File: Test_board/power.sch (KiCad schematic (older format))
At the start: 22 parts, among them J10 4.19mmBananaJack, J11 4.19mmBananaJack, J12 4.19mmBananaJack, J13 4.19mmBananaJack, J14 USB_OTG, U3 LT3652, U4 LT3652, U5 LTC3113

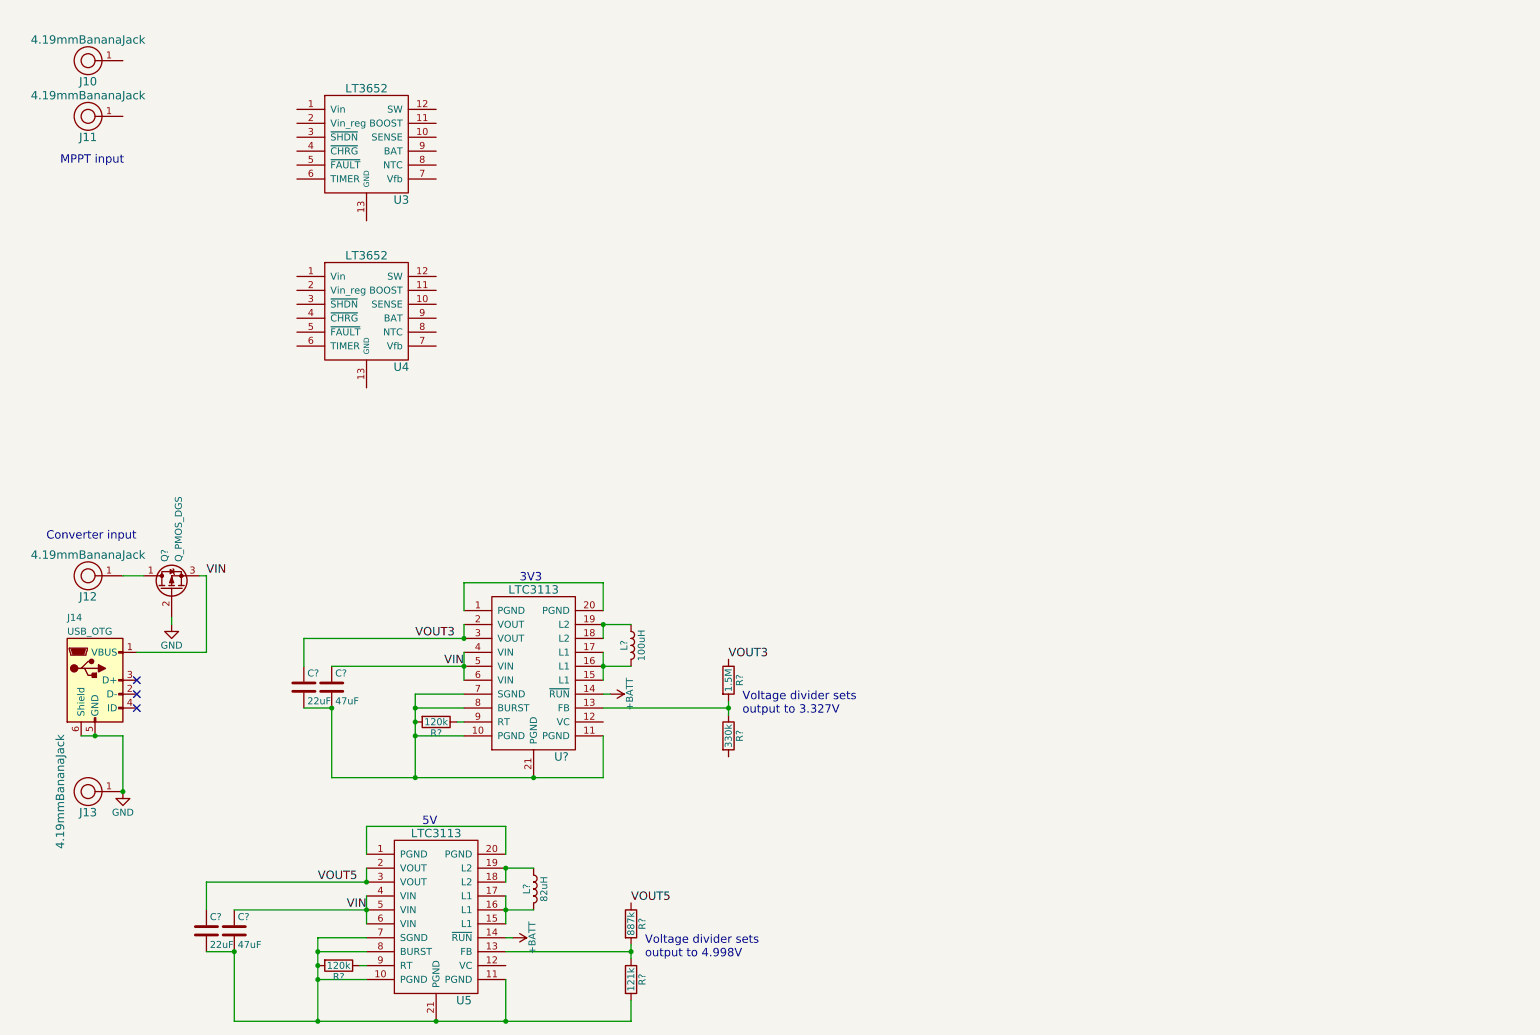
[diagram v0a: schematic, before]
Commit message: Finished schematic
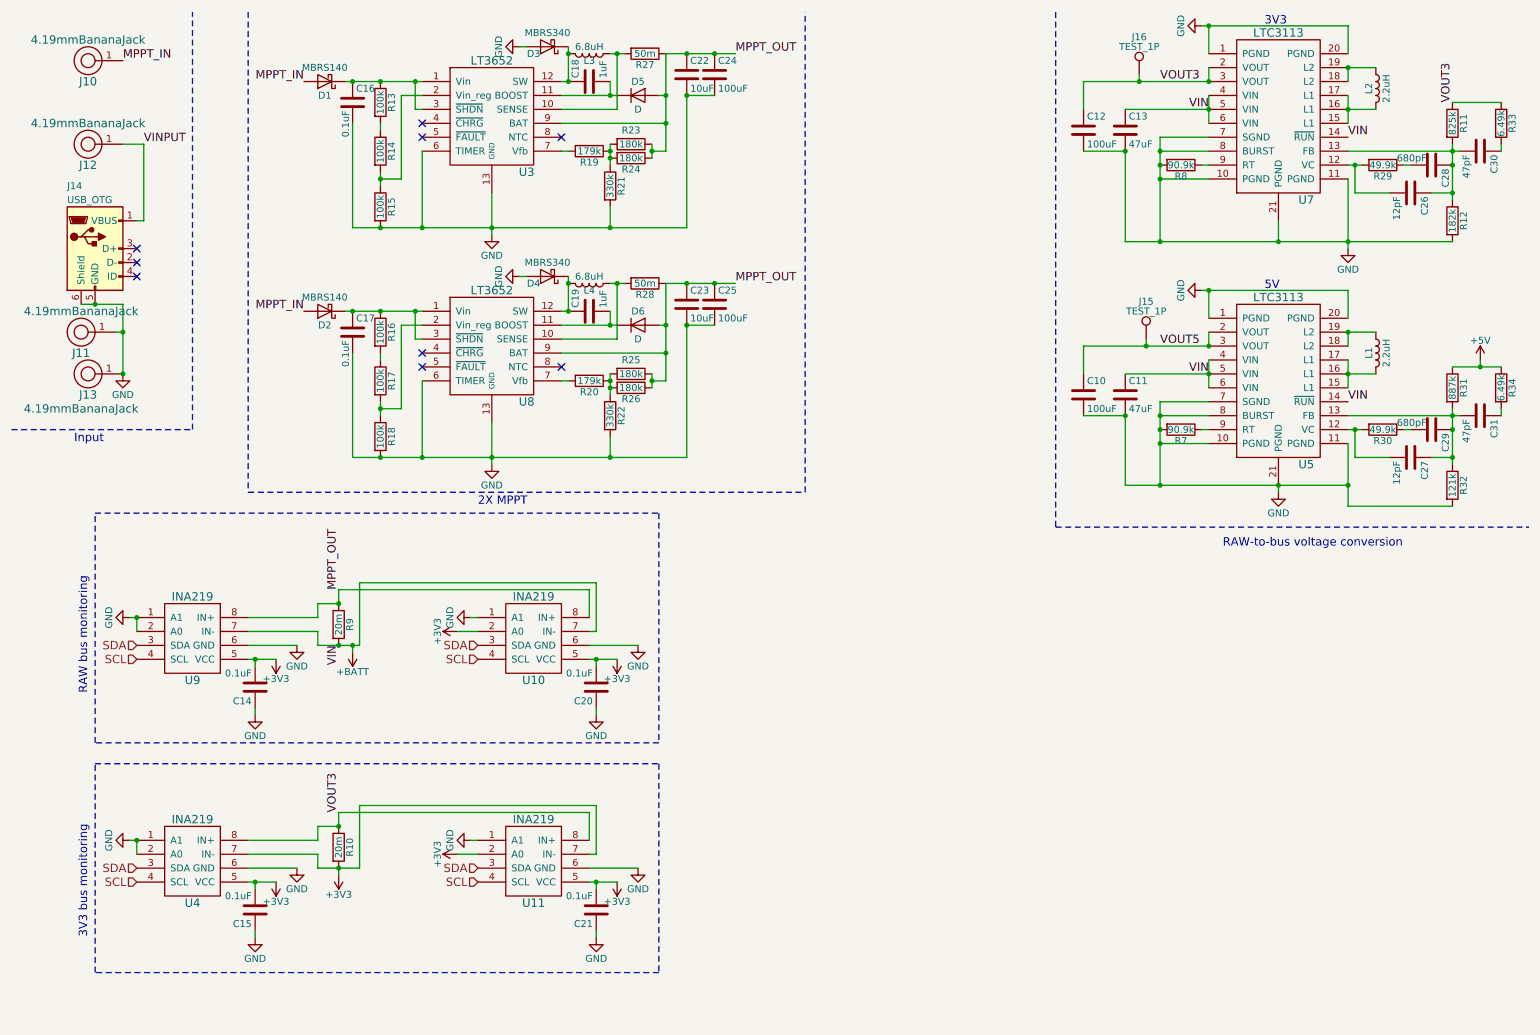
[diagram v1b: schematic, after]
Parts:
- removed Q?: Q_PMOS_DGS, symbol Q_PMOS_DGS
- removed R?: 887k, symbol R
- removed R?: 121k, symbol R
- removed U4: LT3652, symbol LT3652
- added C14, C15, C16, C17, C20, C21: 0.1uF, Capacitors_SMD:C_0805_HandSoldering, symbol C
- added C18, C19: 1uF, symbol C
- added C22, C23: 10uF, symbol C
- added C24, C25: 100uF, symbol C
- added C26, C27: 12pF, symbol C
- added C28, C29: 680pF, symbol C
- added C30, C31: 47pF, symbol C
- added D1, D2: MBRS140, symbol D_Schottky
- added D3, D4: MBRS340, symbol D_Schottky
- added D5, D6: D, symbol D
- added J15, J16: TEST_1P, Measurement_Points:Measurement_Point_Round-SMD-Pad_Big, symbol TEST_1P
- added L3, L4: 6.8uH, symbol L
- added R10, R9: 20m, symbol R
- added R13, R14, R15, R16, R17, R18: 100k, symbol R
- added R19, R20: 179k, symbol R
- added R21, R22: 330k, symbol R
- added R23, R24, R25, R26: 180k, symbol R
- added R27, R28: 50m, symbol R
- added R29, R30: 49.9k, symbol R
- added R31: 887k, symbol R
- added R32: 121k, symbol R
- added R33, R34: 6.49k, symbol R
- added U10, U11, U4, U9: INA219, symbol INA219
- added U8: LT3652, symbol LT3652
- C10, C12: renamed from C?; value 22uF -> 100uF
- L1: renamed from L?; value 82uH -> 2.2uH
- L2: renamed from L?; value 100uH -> 2.2uH
- R11: renamed from R?; value 1.5M -> 825k
- R12: renamed from R?; value 330k -> 182k
- R7, R8: renamed from R?; value 120k -> 90.9k; footprint 0805 -> (none)
- gave numbers to parts that had none: 3
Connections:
- net +BATT: now also C11.1, C13.1, U5.4 (VIN), U5.5 (VIN), U5.6 (VIN), U7.4 (VIN), U7.5 (VIN), U7.6 (VIN), R9.2, U10.7 (IN-), U9.7 (IN-)
- net GND: now also C10.2, C11.2, C12.2, C13.2, J11.1, R12.2, R7.2, R8.2, U3.13 (GND), U3.6 (TIMER), U5.1 (PGND), U5.10 (PGND), U5.11 (PGND), U5.20 (PGND), U5.21 (PGND), U5.7 (SGND), U5.8 (BURST), U7.1 (PGND), U7.10 (PGND), U7.11 (PGND), U7.20 (PGND), U7.21 (PGND), U7.7 (SGND), U7.8 (BURST), C14.1, C15.1, C16.2, C17.2, C20.1, C21.1, C22.2, C23.2, C24.2, C25.2, D3.2 (A), D4.2 (A), R15.2, R18.2, R21.2, R22.2, R32.2, U10.1 (A1), U10.6 (GND), U11.1 (A1), U11.6 (GND), U4.1 (A1), U4.2 (A0), U4.6 (GND), U8.13 (GND), U8.6 (TIMER), U9.1 (A1), U9.2 (A0), U9.6 (GND)
- net VOUT3: now also J16.1, R10.1, R33.1, U11.8 (IN+), U4.8 (IN+)
- net VOUT5: now also J15.1
- net MPPT_IN: now reaches J10.1
- net MPPT_IN: now also D1.2 (A), D2.2 (A)
- net VINPUT: now reaches J12.1
- net VINPUT: now also J14.1 (VBUS)
- net at U3.1 (Vin): now also U3.3 (~SHDN), C16.1, D1.1 (K), R13.1
- net at U3.10 (SENSE): now also L3.1, R27.2
- net at U3.11 (BOOST): now also C18.2, D5.1 (K)
- net at U3.12 (SW): now also C18.1, D3.1 (K), L3.2
- net at U3.2 (Vin_reg): now also R14.2, R15.1
- net at U3.7 (Vfb): now also R19.2
- net MPPT_OUT: now reaches U3.9 (BAT)
- net MPPT_OUT: now also C22.1, C23.1, C24.1, C25.1, D5.2 (A), D6.2 (A), R23.1, R24.1, R25.1, R26.1, R27.1, R28.1, R9.1, U10.8 (IN+), U8.9 (BAT), U9.8 (IN+)
- net at U5.12 (VC): now also C27.2, R30.2
- net at U5.13 (FB): now also C27.1, C29.1, C31.2, R31.2, R32.1
- net at U7.12 (VC): now also C26.2, R29.2
- net at R11.2, R12.1, U7.13 (FB): now also C26.1, C28.1, C30.2
- removed net VIN: C11.1, C13.1, J14.1 (VBUS), U5.4 (VIN), U5.5 (VIN), U5.6 (VIN), U7.4 (VIN), U7.5 (VIN), U7.6 (VIN)
- new net: C28.2, R29.1
- new net: C30.1, R33.2
- new net: C29.2, R30.1
- new net: C31.1, R34.2
- new net: R13.2, R14.1
- new net: R19.1, R21.1, R23.2, R24.2
- new net: C17.1, D2.1 (K), R16.1, U8.1 (Vin), U8.3 (~SHDN)
- new net: L4.1, R28.2, U8.10 (SENSE)
- new net: C19.2, D6.1 (K), U8.11 (BOOST)
- new net: C19.1, D4.1 (K), L4.2, U8.12 (SW)
- new net: R17.2, R18.1, U8.2 (Vin_reg)
- new net: R20.2, U8.7 (Vfb)
- new net: R16.2, R17.1
- new net: R20.1, R22.1, R25.2, R26.2
- new net +3V3: C14.2, C15.2, C20.2, C21.2, R10.2, U10.2 (A0), U10.5 (VCC), U11.2 (A0), U11.5 (VCC), U11.7 (IN-), U4.5 (VCC), U4.7 (IN-), U9.5 (VCC)
- new net +5V: R31.1, R34.1
- new net SCL: U10.4 (SCL), U11.4 (SCL), U4.4 (SCL), U9.4 (SCL)
- new net SDA: U10.3 (SDA), U11.3 (SDA), U4.3 (SDA), U9.3 (SDA)
- no-connect marks 3 -> 9
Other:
- note added: "2X MPPT"
- note added: "3V3 bus monitoring"
- note added: "Input"
- note added: "RAW bus monitoring"
- note added: "RAW-to-bus voltage conversion"
- note removed: "Converter input"
- note removed: "MPPT input"
- note removed: "Voltage divider sets\noutput to 3.327V"
- note removed: "Voltage divider sets\noutput to 4.998V"
- moved on the sheet: C10, C11, C12, C13, J11, J12, J13, J14, L1, L2, R11, R12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
